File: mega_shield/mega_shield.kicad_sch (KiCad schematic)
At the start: 0 parts

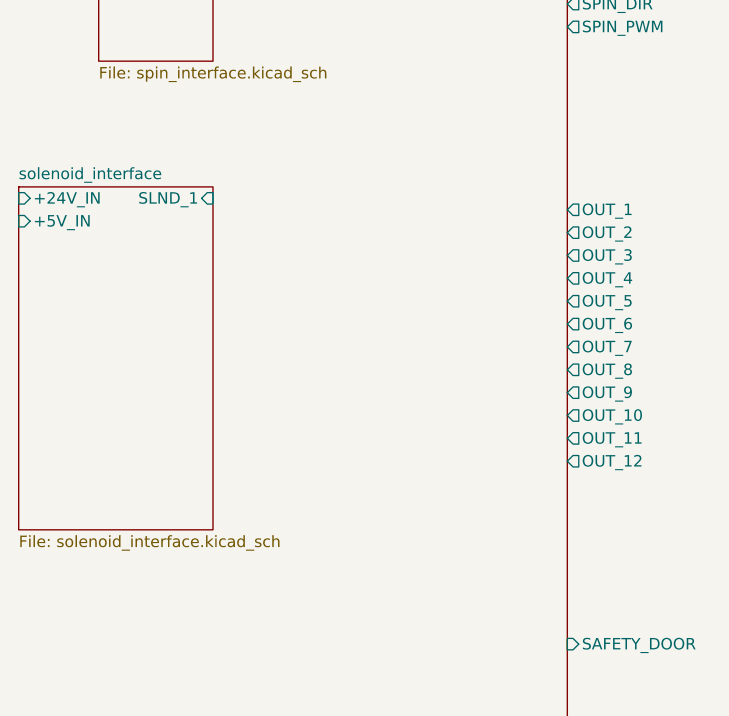
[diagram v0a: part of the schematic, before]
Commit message: Added sheet labels for channels 1-10 to the solenoid interface sheet. Imported pins.
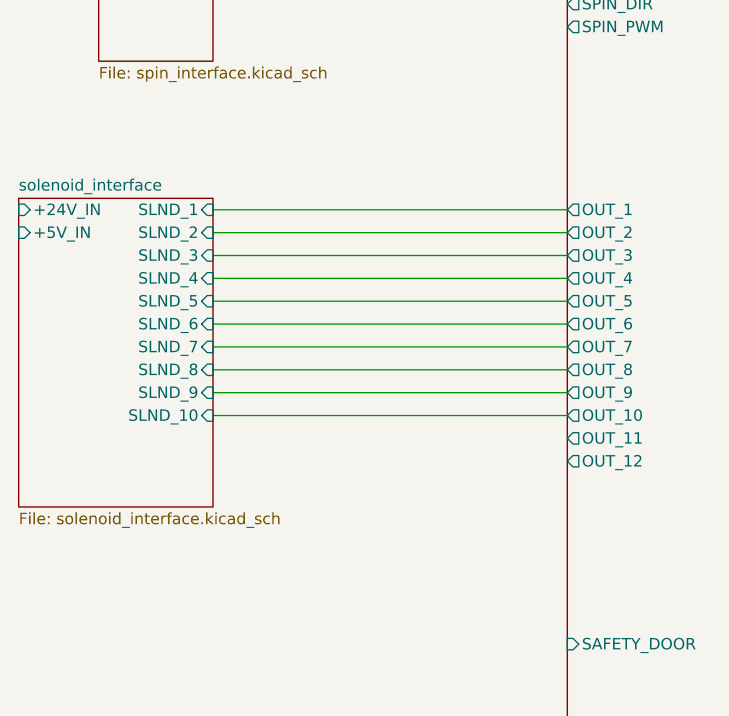
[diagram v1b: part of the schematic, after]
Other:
- sheet solenoid_interface ports: added SLND_10, SLND_2, SLND_3, SLND_4, SLND_5, SLND_6, SLND_7, SLND_8, SLND_9; removed none
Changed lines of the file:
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@@
+	(wire
+		(pts
+			(xy 203.2 124.46) (xy 242.57 124.46)
+		)
+		(stroke
+			(width 0)
+			(type default)
+		)
+	)
 	(wire
 		(pts
@@
 	(wire
 		(pts
+			(xy 203.2 139.7) (xy 242.57 139.7)
+		)
+		(stroke
+			(width 0)
+			(type default)
+		)
+	)
+	(wire
+		(pts
+			(xy 203.2 116.84) (xy 242.57 116.84)
+		)
+		(stroke
+			(width 0)
+			(type default)
+		)
+	)
+	(wire
+		(pts
 			(xy 306.07 104.14) (xy 342.9 104.14)
 		)
@@
 	(wire
 		(pts
+			(xy 203.2 119.38) (xy 242.57 119.38)
+		)
+		(stroke
+			(width 0)
+			(type default)
+		)
+	)
+	(wire
+		(pts
 			(xy 306.07 124.46) (xy 342.9 124.46)
 		)
@@
 	(wire
 		(pts
+			(xy 203.2 127) (xy 242.57 127)
+		)
+		(stroke
+			(width 0)
+			(type default)
+		)
+	)
+	(wire
+		(pts
 			(xy 381 165.1) (xy 364.49 165.1)
 		)
@@
 	(wire
 		(pts
+			(xy 203.2 121.92) (xy 242.57 121.92)
+		)
+		(stroke
+			(width 0)
+			(type default)
+		)
+	)
+	(wire
+		(pts
 			(xy 306.07 172.72) (xy 342.9 172.72)
 		)
@@
 	(wire
 		(pts
+			(xy 203.2 134.62) (xy 242.57 134.62)
+		)
+		(stroke
+			(width 0)
+			(type default)
+		)
+	)
+	(wire
+		(pts
 			(xy 381 83.82) (xy 381 104.14)
 		)
@@
 	(wire
 		(pts
+			(xy 203.2 132.08) (xy 242.57 132.08)
+		)
+		(stroke
+			(width 0)
+			(type default)
+		)
+	)
+	(wire
+		(pts
 			(xy 364.49 83.82) (xy 381 83.82)
 		)
@@
 	(wire
 		(pts
+			(xy 203.2 137.16) (xy 242.57 137.16)
+		)
+		(stroke
+			(width 0)
+			(type default)
+		)
+	)
+	(wire
+		(pts
 			(xy 306.07 121.92) (xy 342.9 121.92)
+		)
+		(stroke
+			(width 0)
+			(type default)
+		)
+	)
+	(wire
+		(pts
+			(xy 203.2 129.54) (xy 242.57 129.54)
 		)
 		(stroke
@@
 	)
 	(sheet
-		(at 181.61 114.3)
-		(size 21.59 38.1)
+		(at 181.61 115.57)
+		(size 21.59 34.29)
 		(exclude_from_sim no)
 		(in_bom yes)
@@
 		)
 		(property "Sheetname" "solenoid_interface"
-			(at 181.61 113.5884 0)
+			(at 181.61 114.8584 0)
 			(effects
 				(font
@@
 		)
 		(property "Sheetfile" "solenoid_interface.kicad_sch"
-			(at 181.61 152.9846 0)
+			(at 181.61 150.4446 0)
 			(effects
 				(font
@@
 		)
 		(pin "+5V_IN" input
-			(at 181.61 118.11 180)
+			(at 181.61 119.38 180)
 			(effects
 				(font
@@
 		)
 		(pin "+24V_IN" input
-			(at 181.61 115.57 180)
+			(at 181.61 116.84 180)
 			(effects
 				(font
@@
 		)
 		(pin "SLND_1" input
-			(at 203.2 115.57 0)
-			(effects
-				(font
+			(at 203.2 116.84 0)
+			(effects
+				(font
+					(size 1.27 1.27)
+				)
+				(justify right)
+			)
+		)
+		(pin "SLND_2" input
+			(at 203.2 119.38 0)
+			(effects
+				(font
+					(size 1.27 1.27)
+				)
+				(justify right)
+			)
+		)
+		(pin "SLND_3" input
+			(at 203.2 121.92 0)
+			(effects
+				(font
+					(size 1.27 1.27)
+				)
+				(justify right)
+			)
+		)
+		(pin "SLND_4" input
+			(at 203.2 124.46 0)
+			(effects
+				(font
+					(size 1.27 1.27)
+				)
+				(justify right)
+			)
+		)
+		(pin "SLND_5" input
+			(at 203.2 127 0)
+			(effects
+				(font
+					(size 1.27 1.27)
+				)
+				(justify right)
+			)
+		)
+		(pin "SLND_6" input
+			(at 203.2 129.54 0)
+			(effects
+				(font
+					(size 1.27 1.27)
+				)
+				(justify right)
+			)
+		)
+		(pin "SLND_7" input
+			(at 203.2 132.08 0)
+			(effects
+				(font
+					(size 1.27 1.27)
+				)
+				(justify right)
+			)
+		)
+		(pin "SLND_8" input
+			(at 203.2 134.62 0)
+			(effects
+				(font
+					(size 1.27 1.27)
+				)
+				(justify right)
+			)
+		)
+		(pin "SLND_9" input
+			(at 203.2 137.16 0)
+			(effects
+				(font
+					(size 1.27 1.27)
+				)
+				(justify right)
+			)
+		)
+		(pin "SLND_10" input
+			(at 203.2 139.7 0)
+			(effects
+				(font
